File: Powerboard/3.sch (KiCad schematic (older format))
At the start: 32 parts

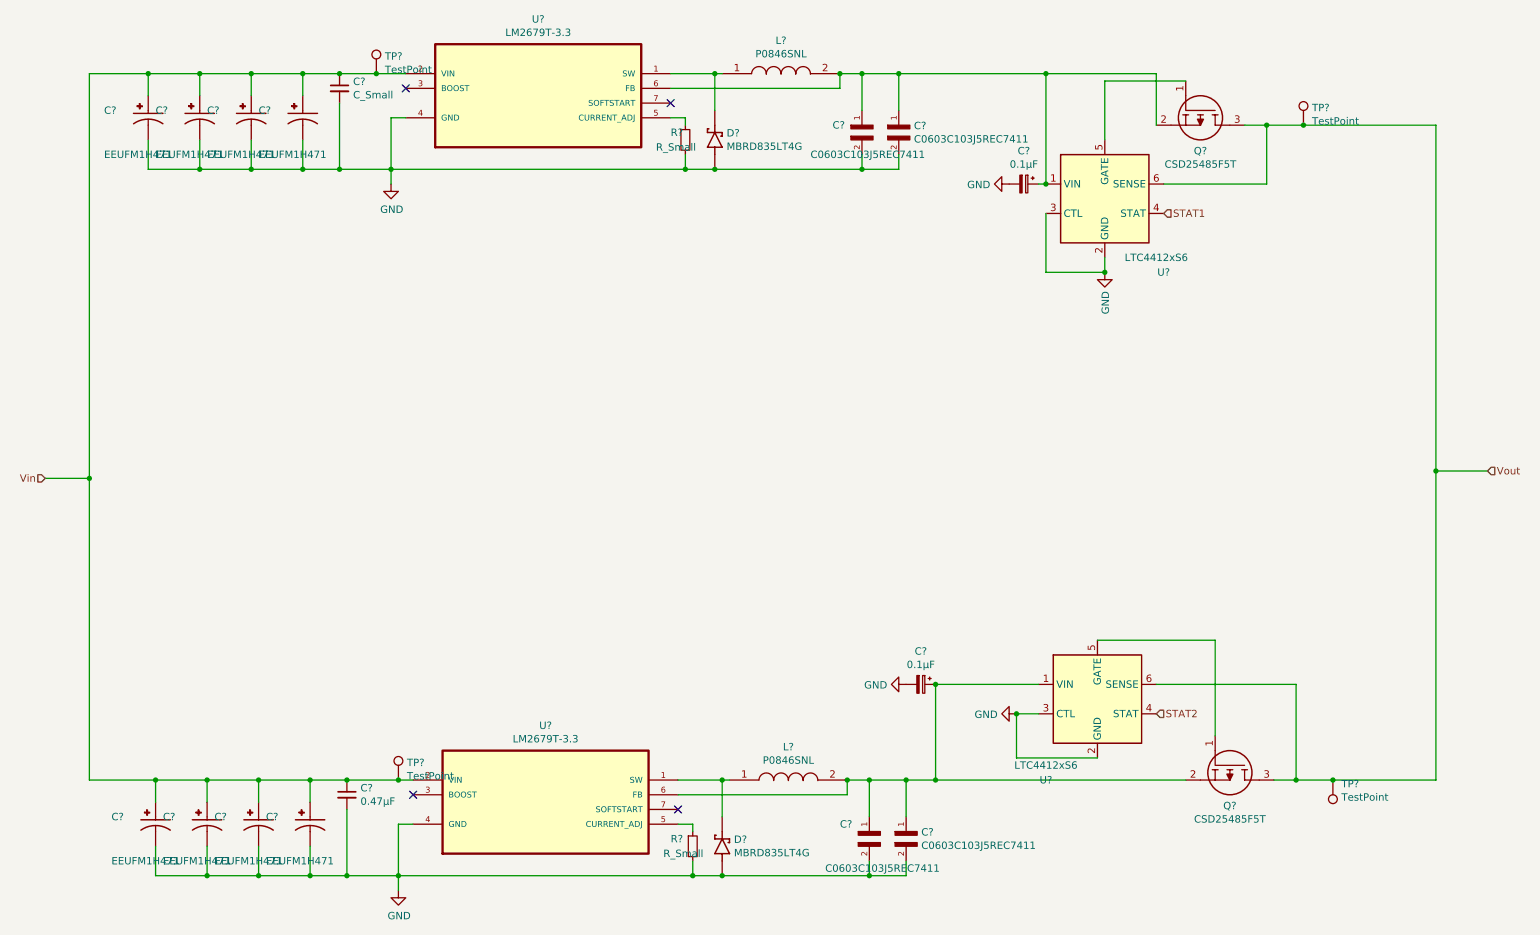
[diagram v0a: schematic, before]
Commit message: 19/02/2022
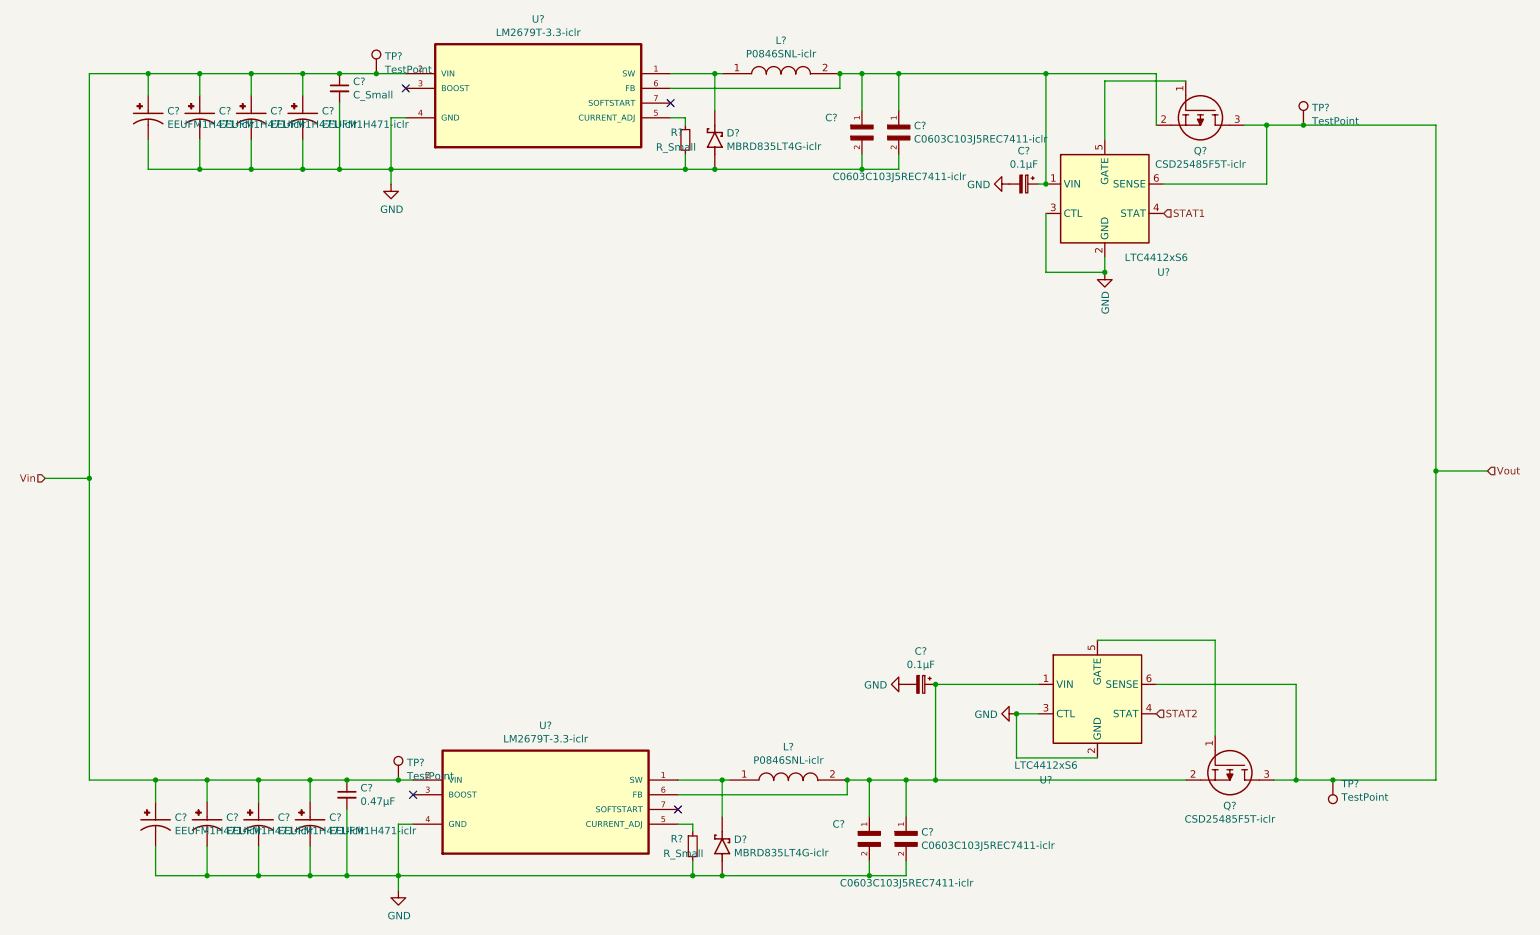
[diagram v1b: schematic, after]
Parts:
- removed C? (x8): EEUFM1H471, CAPPRD500W60D1250H2000, symbol power_new_25012022-rescue:EEUFM1H471-iclr
- removed C? (x4): C0603C103J5REC7411, CAPC1608X87N, symbol power_new_25012022-rescue:C0603C103J5REC7411-iclr
- removed D? (x2): MBRD835LT4G, DPAK229P990X238-3N, symbol power_new_25012022-rescue:MBRD835LT4G-iclr
- removed L? (x2): P0846SNL, P0846SNL, symbol power_new_25012022-rescue:P0846SNL-iclr
- removed Q? (x2): CSD25485F5T, CSD13385F5, symbol power_new_25012022-rescue:CSD25485F5T-iclr
- removed U? (x2): LM2679T-3.3, TO127P457X1016X2052-7P, symbol power_new_25012022-rescue:LM2679T-3.3-iclr
- added C? (x4): C0603C103J5REC7411-iclr, CAPC1608X87N, symbol iclr:C0603C103J5REC7411-iclr
- added C? (x8): EEUFM1H471-iclr, CAPPRD500W60D1250H2000, symbol iclr:EEUFM1H471-iclr
- added D? (x2): MBRD835LT4G-iclr, DPAK229P990X238-3N, symbol iclr:MBRD835LT4G-iclr
- added L? (x2): P0846SNL-iclr, P0846SNL, symbol iclr:P0846SNL-iclr
- added Q? (x2): CSD25485F5T-iclr, CSD13385F5, symbol iclr:CSD25485F5T-iclr
- added U? (x2): LM2679T-3.3-iclr, TO127P457X1016X2052-7P, symbol iclr:LM2679T-3.3-iclr
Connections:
- net GND: now also C?.2, C?.2, C?.2, C?.2, C?.N, C?.N, C?.N, C?.N, C?.N, C?.N, C?.N, C?.N, D?.1, D?.1, D?.3, D?.3, U?.4 (GND), U?.4 (GND)
- net Vin: now also C?.P, C?.P, C?.P, C?.P, C?.P, C?.P, C?.P, C?.P, U?.2 (VIN), U?.2 (VIN)
- net Vout: now also Q?.3, Q?.3
- net at C?.1, U?.1 (VIN): now also C?.1, C?.1, L?.2, Q?.2, U?.6 (FB) (x2)
- net at R?.1: now also U?.5 (CURRENT_ADJ) (x2)
- net at U?.5 (GATE): now also Q?.1 (x2)
- new net: D?.4, L?.1, U?.1 (SW) (x2)
